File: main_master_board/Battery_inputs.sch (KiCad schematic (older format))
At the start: 4 parts

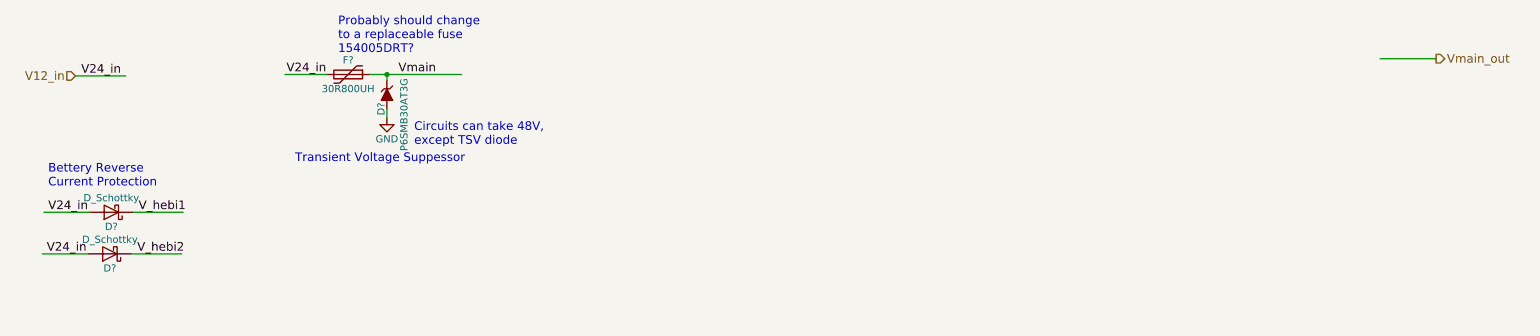
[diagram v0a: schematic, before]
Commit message: Added lots of things. current/voltage monitoring. and other stuff
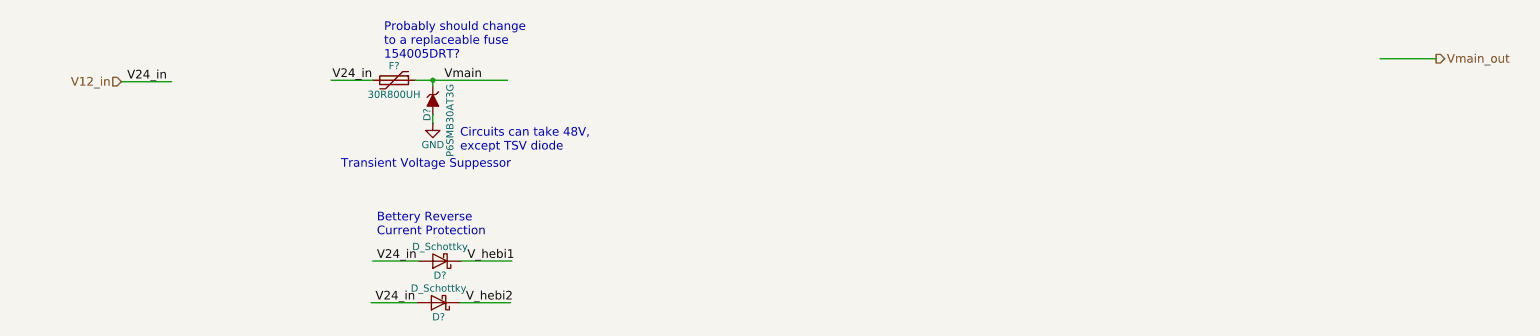
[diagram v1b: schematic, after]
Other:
- moved on the sheet: D?, F?
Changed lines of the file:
@@
 LIBS:FDS4935A
 LIBS:Si1900DL
+LIBS:Amplifiers
+LIBS:Connectors
+LIBS:DataStorage
+LIBS:Diodes
+LIBS:Microprocessors
+LIBS:MiscellaneousDevices
+LIBS:Passives
+LIBS:PMOD
+LIBS:PowerComponents
+LIBS:RepeaterParts
+LIBS:RF_OEM_Parts
 LIBS:Sensors
+LIBS:TransistorParts
 LIBS:LP3852-3.3
 LIBS:0s102011ma1qn1
@@
 L Polyfuse F?
 U 1 1 586EDB59
-P 2820 1270
-F 0 "F?" V 2720 1270 50  0000 C CNN
-F 1 "30R800UH" V 2920 1270 50  0000 C CNN
-F 2 "" H 2870 1070 50  0001 L CNN
-F 3 "http://datasheet.octopart.com/30R800UH-Littelfuse-datasheet-8746242.pdf" H 2820 1270 50  0001 C CNN
-	1    2820 1270
+P 3140 1310
+F 0 "F?" V 3040 1310 50  0000 C CNN
+F 1 "30R800UH" V 3240 1310 50  0000 C CNN
+F 2 "" H 3190 1110 50  0001 L CNN
+F 3 "http://datasheet.octopart.com/30R800UH-Littelfuse-datasheet-8746242.pdf" H 3140 1310 50  0001 C CNN
+	1    3140 1310
 	0    1    1    0
 $EndComp
@@
 L ZENERsmall D?
 U 1 1 586EDB68
-P 3090 1410
-F 0 "D?" H 3190 1370 50  0000 C CNN
-F 1 "P6SMB30AT3G" H 3230 1530 50  0000 C CNN
-F 2 "" H 3090 1410 50  0000 C CNN
-F 3 "http://datasheet.octopart.com/P6SMB36AT3G-ON-Semiconductor-datasheet-5314825.pdf" H 3090 1410 50  0001 C CNN
-	1    3090 1410
+P 3410 1450
+F 0 "D?" H 3510 1410 50  0000 C CNN
+F 1 "P6SMB30AT3G" H 3550 1570 50  0000 C CNN
+F 2 "" H 3410 1450 50  0000 C CNN
+F 3 "http://datasheet.octopart.com/P6SMB36AT3G-ON-Semiconductor-datasheet-5314825.pdf" H 3410 1450 50  0001 C CNN
+	1    3410 1450
 	0    1    1    0
 $EndComp
 Wire Wire Line
-	2970 1270 3610 1270
+	3290 1310 3930 1310
 Wire Wire Line
-	3090 1270 3090 1310
-Connection ~ 3090 1270
+	3410 1310 3410 1350
+Connection ~ 3410 1310
 Wire Wire Line
-	3090 1510 3090 1570
+	3410 1550 3410 1610
 $Comp
 L GND #PWR?
 U 1 1 586EDB74
-P 3090 1570
-F 0 "#PWR?" H 3090 1320 50  0001 C CNN
-F 1 "GND" H 3090 1420 50  0000 C CNN
-F 2 "" H 3090 1570 50  0000 C CNN
-F 3 "" H 3090 1570 50  0000 C CNN
-	1    3090 1570
+P 3410 1610
+F 0 "#PWR?" H 3410 1360 50  0001 C CNN
+F 1 "GND" H 3410 1460 50  0000 C CNN
+F 2 "" H 3410 1610 50  0000 C CNN
+F 3 "" H 3410 1610 50  0000 C CNN
+	1    3410 1610
 	1    0    0    -1
 $EndComp
-Text Notes 2750 1130 0    60   ~ 0
+Text Notes 3070 1170 0    60   ~ 0
 Probably should change \nto a replaceable fuse\n154005DRT?
-Text Notes 2450 1890 0    60   ~ 0
+Text Notes 2770 1930 0    60   ~ 0
 Transient Voltage Suppessor
-Text Label 3170 1270 0    60   ~ 0
+Text Label 3490 1310 0    60   ~ 0
 Vmain
-Text Notes 3280 1770 0    60   ~ 0
+Text Notes 3600 1810 0    60   ~ 0
 Circuits can take 48V, \nexcept TSV diode
-Text HLabel 920  1280 0    60   Input ~ 0
+Text HLabel 1240 1320 0    60   Input ~ 0
 V12_in
 Text HLabel 10400 1160 2    60   Output ~ 0
@@
 L D_Schottky D?
 U 1 1 586EEE5D
-P 1170 2230
-F 0 "D?" H 1170 2330 50  0000 C CNN
-F 1 "D_Schottky" H 1170 2130 50  0000 C CNN
-F 2 "DPAK" H 1170 2230 50  0001 C CNN
-F 3 "http://datasheet.octopart.com/STPS5H100B-TR-STMicroelectronics-datasheet-5318140.pdf" H 1170 2230 50  0001 C CNN
-	1    1170 2230
+P 3460 2570
+F 0 "D?" H 3460 2670 50  0000 C CNN
+F 1 "D_Schottky" H 3460 2470 50  0000 C CNN
+F 2 "DPAK" H 3460 2570 50  0001 C CNN
+F 3 "http://datasheet.octopart.com/STPS5H100B-TR-STMicroelectronics-datasheet-5318140.pdf" H 3460 2570 50  0001 C CNN
+	1    3460 2570
 	-1   0    0    1
 $EndComp
 Wire Wire Line
-	920  1280 1270 1280
-Text Label 960  1280 0    60   ~ 0
+	1240 1320 1590 1320
+Text Label 1280 1320 0    60   ~ 0
 V24_in
 Wire Wire Line
-	2670 1270 2380 1270
+	2990 1310 2700 1310
 Wire Wire Line
-	1020 2230 700  2230
+	3310 2570 2990 2570
 Wire Wire Line
-	1320 2230 1670 2230
-Text Label 2390 1270 0    60   ~ 0
+	3610 2570 3960 2570
+Text Label 2710 1310 0    60   ~ 0
 V24_in
-Text Label 730  2230 0    60   ~ 0
+Text Label 3020 2570 0    60   ~ 0
 V24_in
-Text Label 1360 2230 0    60   ~ 0
+Text Label 3650 2570 0    60   ~ 0
 V_hebi1
 $Comp
 L D_Schottky D?
 U 1 1 586EF429
-P 1160 2520
-F 0 "D?" H 1160 2620 50  0000 C CNN
-F 1 "D_Schottky" H 1160 2420 50  0000 C CNN
-F 2 "DPAK" H 1160 2520 50  0001 C CNN
-F 3 "http://datasheet.octopart.com/STPS5H100B-TR-STMicroelectronics-datasheet-5318140.pdf" H 1160 2520 50  0001 C CNN
-	1    1160 2520
+P 3450 2860
+F 0 "D?" H 3450 2960 50  0000 C CNN
+F 1 "D_Schottky" H 3450 2760 50  0000 C CNN
+F 2 "DPAK" H 3450 2860 50  0001 C CNN
+F 3 "http://datasheet.octopart.com/STPS5H100B-TR-STMicroelectronics-datasheet-5318140.pdf" H 3450 2860 50  0001 C CNN
+	1    3450 2860
 	-1   0    0    1
 $EndComp
 Wire Wire Line
-	1010 2520 690  2520
+	3300 2860 2980 2860
 Wire Wire Line
-	1310 2520 1660 2520
-Text Label 720  2520 0    60   ~ 0
+	3600 2860 3950 2860
+Text Label 3010 2860 0    60   ~ 0
 V24_in
-Text Label 1350 2520 0    60   ~ 0
+Text Label 3640 2860 0    60   ~ 0
 V_hebi2
-Text Notes 730  2060 0    60   ~ 0
+Text Notes 3020 2400 0    60   ~ 0
 Bettery Reverse\nCurrent Protection
 $EndSCHEMATC
